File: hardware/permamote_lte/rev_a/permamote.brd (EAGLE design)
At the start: 27 x 60 mm, 116 parts, among them IC1 NRF9160, J1 TC2030-JLINK-NL, J2 U.FL-R-SMT, J3 NANO_SIM, J4 U.FL-R-SMT, J5 DM3AT-SF-PEJM5, Q1 PMDXB950UPEL, Q10 PMDXB950UPEL, Q2 PMDXB950UPEL, Q3 PMDXB950UPEL, Q4 PMDXB950UPEL, Q5 PMDXB950UPEL, Q6 PMDXB950UPEL, Q7 PMDXB950UPEL, Q8 PMDXB950UPEL, U1 AB1815-T3, U10 SIP32510, U11 SI7021-A20-GM1, U12 TCS34725, U13 TPD3F303DPVR, U2 BQ25505, U3 EKMB1101111, U4 BGA725L6, U6 LIS2DW12, U7 MAX17222, U8 MAX44009, U9 MS5637-02BA03, X4 ABS07-32.768KHZ-7-T

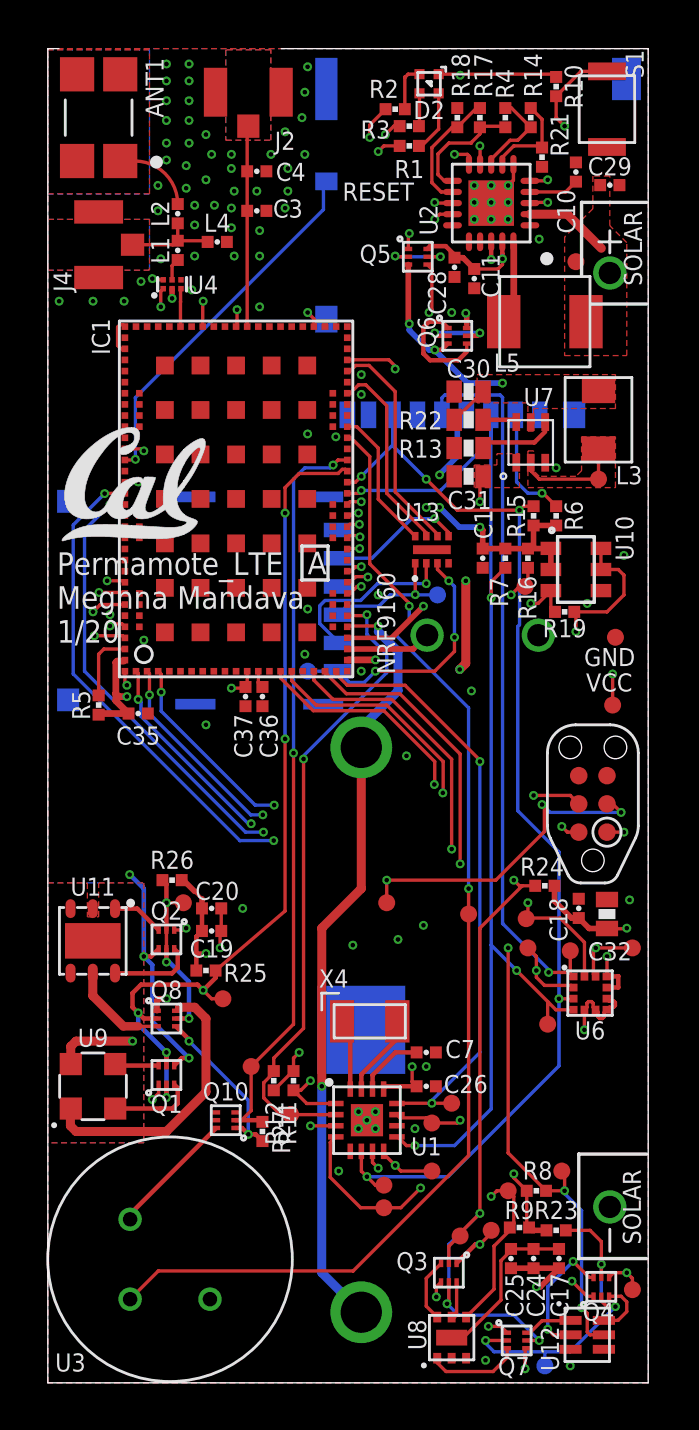
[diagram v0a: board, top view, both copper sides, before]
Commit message: cleaned up wirestubs
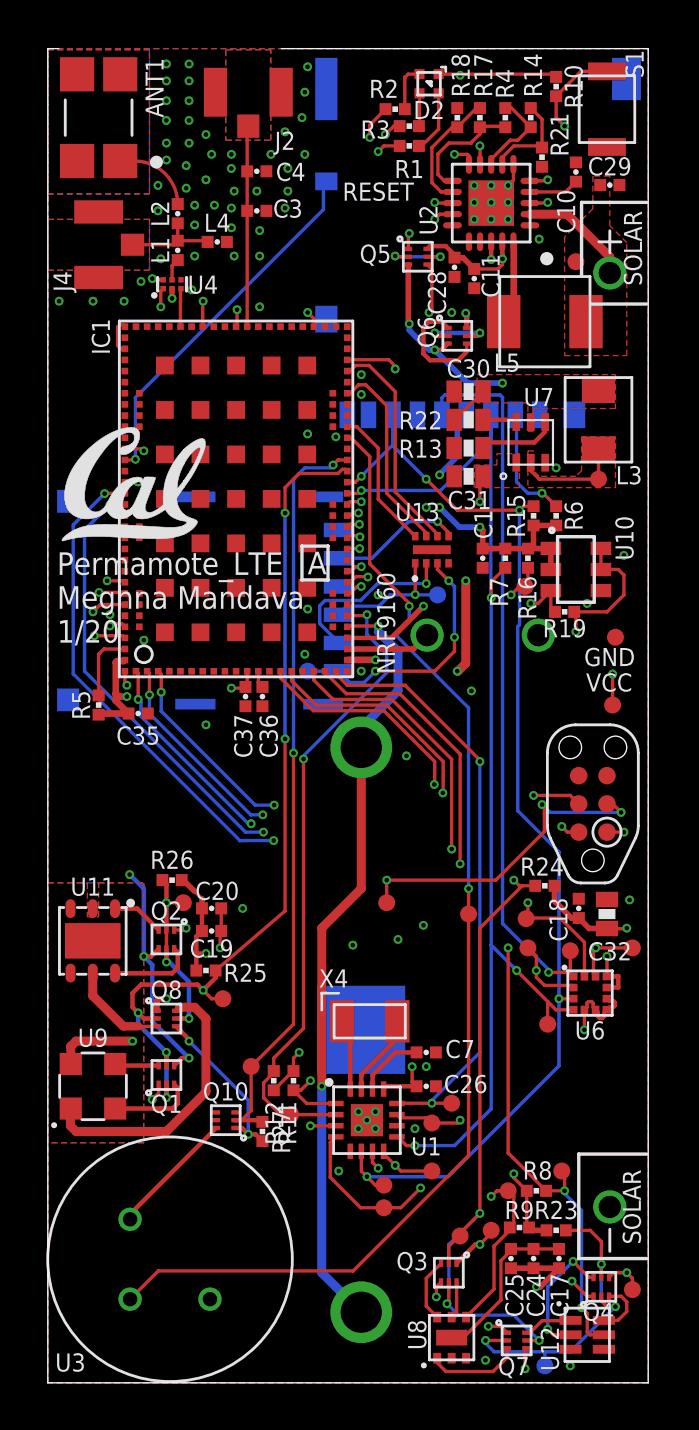
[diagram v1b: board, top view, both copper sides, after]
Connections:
- net GND: now also U13.9
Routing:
- net MISO: track 53.9 -> 52.4 mm
- net GND: track 31.9 -> 30.6 mm
- net VSOL: track 27.3 -> 28.5 mm
- net LBST: track 4.61 -> 3.79 mm
- net VCC: track 62.4 -> 61.7 mm

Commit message: replaced parts with correct library
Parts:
- ANT1: device 1462350001:ANT_1462350001 -> chips:ANT_1462350001
- IC1: device nRF9160:NRF9160 -> chips:NRF9160
- U13: device TPD3F303:DPV8_1P7X0P4 -> chips:DPV8_1P7X0P4
- U4: device Particle:LNA-TSLP-6-2-ORIG -> chips:LNA-TSLP-6-2-ORIG
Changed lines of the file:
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@@
 <attribute name="NAME" x="0.254" y="49.53" size="0.8128" layer="25" font="vector" ratio="12" rot="R270" align="bottom-center"/>
 </element>
-<element name="ANT1" library="1462350001" package="ANT_1462350001" value="1462350001" x="2.286" y="56.896" smashed="yes" rot="R90">
+<element name="ANT1" library="chips" package="ANT_1462350001" value="1462350001" x="2.286" y="56.896" smashed="yes" rot="R90">
 <attribute name="DESCRIPTION" value=" Antenna GPS 1.4dBi Gain 1578MHz SMD T/R " x="2.286" y="56.896" size="1.778" layer="27" rot="R90" display="off"/>
 <attribute name="DIGI-KEY_PART_NUMBER" value="WM15009CT-ND" x="2.286" y="56.896" size="1.778" layer="27" rot="R90" display="off"/>
@@
 <attribute name="NAME" x="11.938" y="9.398" size="1.778" layer="22" font="vector" ratio="12" rot="MR90"/>
 </element>
-<element name="IC1" library="nRF9160" package="NRF9160" value="NRF9160" x="13.716" y="31.75" smashed="yes" rot="R90">
+<element name="IC1" library="chips" package="NRF9160" value="NRF9160" x="13.716" y="31.75" smashed="yes" rot="R90">
 <attribute name="NAME" x="2.794" y="46.228" size="0.8128" layer="25" font="vector" ratio="12" rot="R90"/>
 <attribute name="VALUE" x="15.621" y="31.877" size="0.8128" layer="25" font="vector" ratio="12" rot="R90"/>
@@
 <attribute name="NAME" x="10.922" y="54.864" size="0.8128" layer="25" font="vector" ratio="12" rot="R180" align="bottom-center"/>
 </element>
-<element name="U4" library="Particle" package="LNA-TSLP-6-2-ORIG" value="BGA725L6" x="5.588" y="49.403" smashed="yes" rot="R90">
+<element name="U4" library="chips" package="LNA-TSLP-6-2-ORIG" value="BGA725L6" x="5.588" y="49.403" smashed="yes" rot="R90">
 <attribute name="NAME" x="7.663" y="49.792" size="0.8128" layer="25" font="vector" ratio="12" rot="R180"/>
 <attribute name="VALUE" x="6.388" y="48.903" size="0.5" layer="27" rot="R90" align="top-left"/>
@@
 <element name="TP31" library="headers" package="PAD.03X.03" value="TEST-POINT" x="11.684" y="32.004" smashed="yes" rot="MR270"/>
 <element name="TP32" library="headers" package="PAD.03X.03" value="TEST-POINT" x="21.463" y="35.814" smashed="yes"/>
-<element name="U13" library="TPD3F303" package="DPV8_1P7X0P4" value="TPD3F303DPVR" x="17.272" y="37.465" smashed="yes" rot="R90">
+<element name="U13" library="chips" package="DPV8_1P7X0P4" value="TPD3F303DPVR" x="17.272" y="37.465" smashed="yes" rot="R90">
 <attribute name="MANUFACTURER_PART_NUMBER" value="TPD3F303DPVR" x="17.272" y="37.465" size="1.778" layer="27" rot="R90" display="off"/>
 <attribute name="NAME" x="15.621" y="38.7604" size="0.8128" layer="25" font="vector" ratio="12" rot="SR0"/>
